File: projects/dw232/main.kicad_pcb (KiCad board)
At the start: 4 copper layers, 27 parts, among them P101 CONN_01X07, Q501 MMBT3904, Q502 MMBT3904, U501 LM741, U502 LM741, U503 2DW232

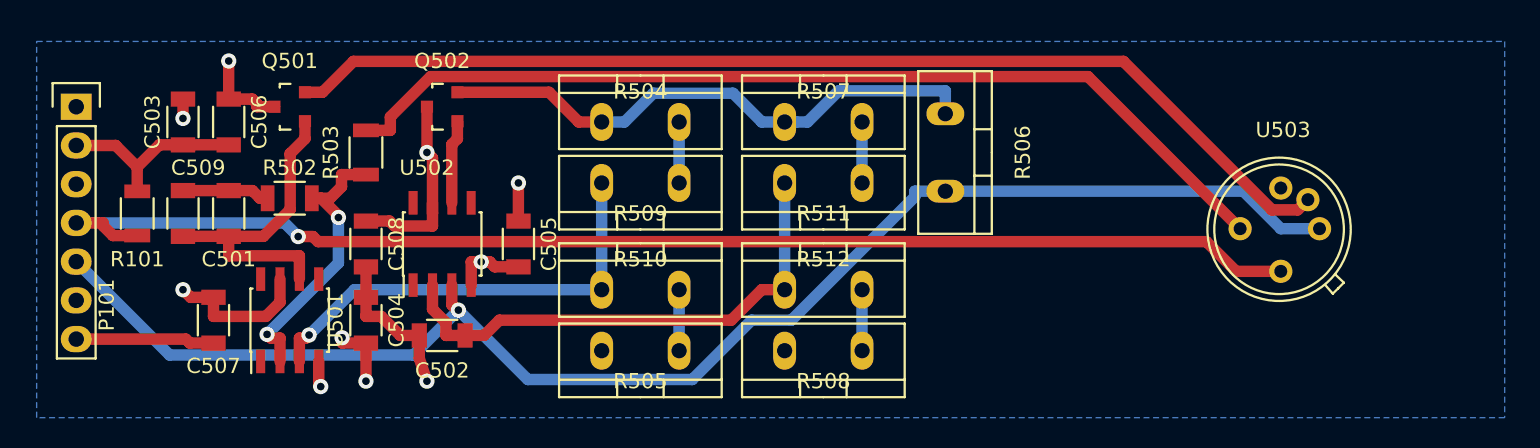
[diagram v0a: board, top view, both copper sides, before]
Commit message: fix front and back silk
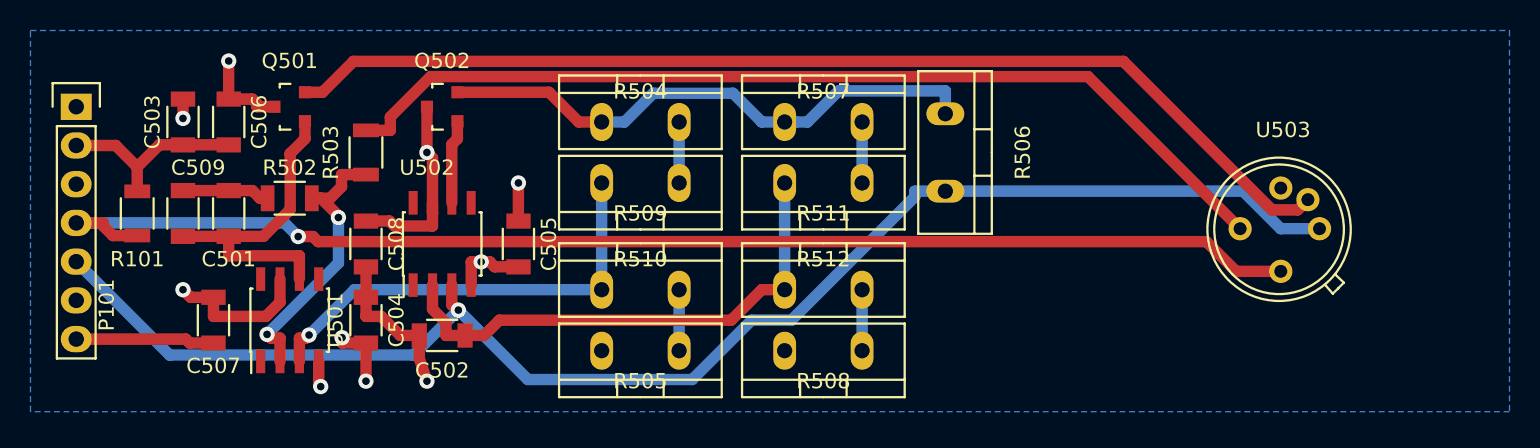
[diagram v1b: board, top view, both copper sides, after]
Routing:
- added copper zone on In1.Cu, net AGND
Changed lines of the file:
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@@
   (general
     (links 52)
-    (no_connects 7)
-    (area 42 29 138.684001 54.394001)
+    (no_connects 0)
+    (area 42 29 139.000001 54.000001)
     (thickness 1.6)
     (drawings 0)
@@
   (layers
     (0 F.Cu signal)
-    (1 In1.Cu signal)
+    (1 In1.Cu signal hide)
     (2 In2.Cu signal hide)
     (31 B.Cu signal hide)
@@
     (36 B.SilkS user hide)
     (37 F.SilkS user hide)
-    (38 B.Mask user hide)
+    (38 B.Mask user)
     (39 F.Mask user hide)
-    (40 Dwgs.User user)
+    (40 Dwgs.User user hide)
     (41 Cmts.User user)
     (42 Eco1.User user)
@@
   (segment (start 63.2433 46) (end 60.27 48.9733) (width 0.75) (layer B.Cu) (net 18))
   (segment (start 79.46 46) (end 63.2433 46) (width 0.75) (layer B.Cu) (net 18) (status 10))
+  (zone (net 0) (net_name "") (layer F.Mask) (hatch edge 0.508)
+    (connect_pads (clearance 0.508))
+    (min_thickness 0.254)
+    (fill yes (arc_segments 16) (thermal_gap 0.508) (thermal_bridge_width 0.508))
+    (polygon
+      (pts
+        (xy 139 54) (xy 42 54) (xy 42 29) (xy 139 29)
+      )
+    )
+  )
+  (zone (net 15) (net_name AGND) (layer In1.Cu) (hatch edge 0.508)
+    (connect_pads (clearance 0.508))
+    (min_thickness 0.254)
+    (fill yes (arc_segments 16) (thermal_gap 0.508) (thermal_bridge_width 0.508))
+    (polygon
+      (pts
+        (xy 139 54) (xy 42 54) (xy 42 29) (xy 139 29)
+      )
+    )
+  )
   (zone (net 1) (net_name +VE) (layer In2.Cu) (hatch edge 0.508)
     (connect_pads (clearance 0.508))
@@
     (polygon
       (pts
-        (xy 138.684 54.394) (xy 42.402 54.394) (xy 42.402 29.718) (xy 138.684 29.718)
+        (xy 139 54) (xy 42 54) (xy 42 29) (xy 139 29)
       )
     )
@@
     (polygon
       (pts
-        (xy 138.684 54.394) (xy 42.402 54.394) (xy 42.402 29.718) (xy 138.684 29.718)
+        (xy 139 54) (xy 42 54) (xy 42 29) (xy 139 29)
       )
     )
   )
-  (zone (net 0) (net_name "") (layer F.Mask) (hatch edge 0.508)
+  (zone (net 0) (net_name "") (layer B.Mask) (hatch edge 0.508)
     (connect_pads (clearance 0.508))
     (min_thickness 0.254)
@@
     (polygon
       (pts
-        (xy 129 54) (xy 42 54) (xy 42 29) (xy 129 29)
+        (xy 139 54) (xy 42 54) (xy 42 29) (xy 139 29)
       )
     )
